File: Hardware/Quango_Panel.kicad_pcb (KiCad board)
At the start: 2 copper layers, 81 x 128.5 mm, 43 parts

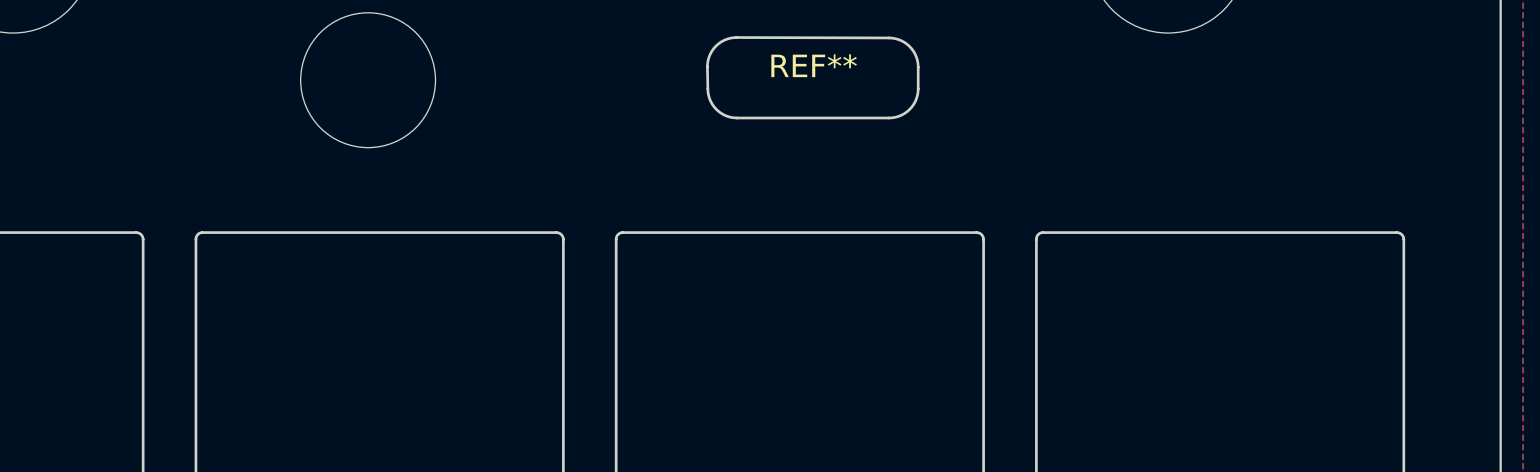
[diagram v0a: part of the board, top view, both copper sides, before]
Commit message: Final Updates for v1.0 production
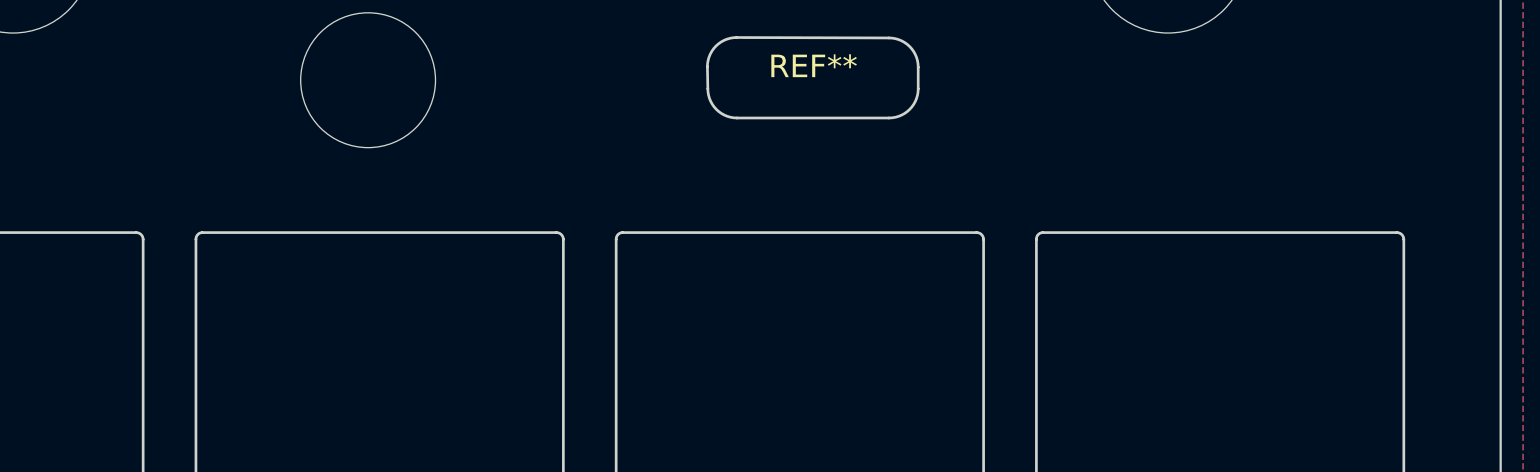
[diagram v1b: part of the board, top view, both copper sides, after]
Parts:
- removed kibuzzard-646A4AD3: G***, kibuzzard-646A4AD3
- removed kibuzzard-646A4ADD: G***, kibuzzard-646A4ADD
- removed kibuzzard-646A4AF9: G***, kibuzzard-646A4AF9
- removed kibuzzard-646B76FE: G***, kibuzzard-646B76FE
- removed kibuzzard-646B7712: G***, kibuzzard-646B7712
- removed kibuzzard-646B771E: G***, kibuzzard-646B771E
- removed kibuzzard-646B9F04: G***, kibuzzard-646B9F04
- removed kibuzzard-646B9FB5: G***, kibuzzard-646B9FB5
- removed kibuzzard-646BA02D: G***, kibuzzard-646BA02D
- added kibuzzard-646C865B: G***, kibuzzard-646C865B, F.Cu at (90.5, 124.4)
- added kibuzzard-646C8A92: G***, kibuzzard-646C8A92, F.Cu at (54.3, 96.1)
- added kibuzzard-646C8AA8: G***, kibuzzard-646C8AA8, F.Cu at (54.3, 73.4)
- added kibuzzard-646C8AB8: G***, kibuzzard-646C8AB8, F.Cu at (54.3, 118.5)
- added kibuzzard-646C8AC0: G***, kibuzzard-646C8AC0, F.Cu at (54.6, 50.8)
- added kibuzzard-646C8AF5: G***, kibuzzard-646C8AF5, F.Cu at (126.2, 50.9)
- added kibuzzard-646C8AFB: G***, kibuzzard-646C8AFB, F.Cu at (126.5, 73.6)
- added kibuzzard-646C8B02: G***, kibuzzard-646C8B02, F.Cu at (126.5, 95.9)
- added kibuzzard-646C8B09: G***, kibuzzard-646C8B09, F.Cu at (126.5, 118.6)
- moved kibuzzard-646BA8C3 0.40 mm to (82.2, 150.6)
- moved kibuzzard-646BA8CA 0.40 mm to (98.8, 150.6)
